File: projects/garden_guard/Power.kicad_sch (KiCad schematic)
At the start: 50 parts, among them IC1 ACPL-227-50CE, IC2 INA226AQDGSRQ1, IC3 INA226AQDGSRQ1, J7 USB_C_Receptacle_USB2.0, U10 TPS2121RUXR, U11 MAX20408AFOF, U9 Ag5810

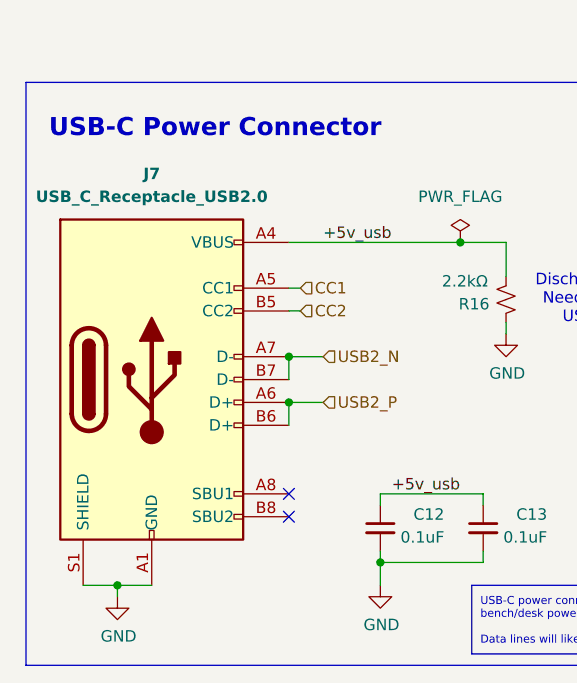
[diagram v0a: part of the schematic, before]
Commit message: - Still working through DRC - Minor board setup tweaks
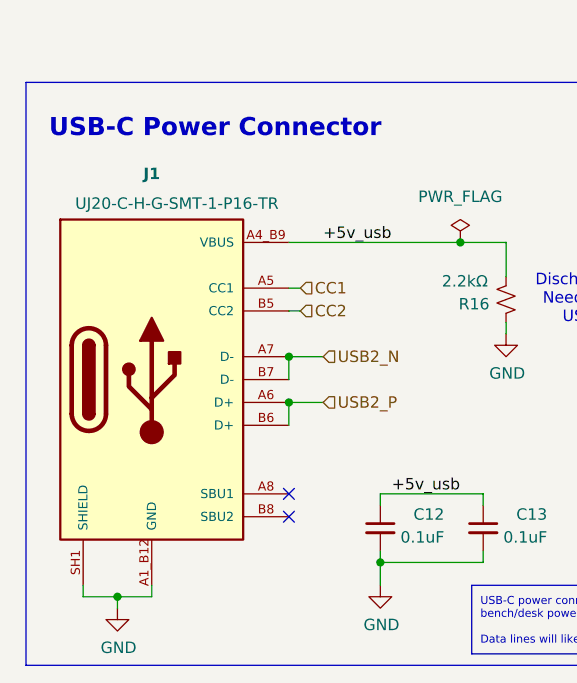
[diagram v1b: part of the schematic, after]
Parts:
- removed J7: USB_C_Receptacle_USB2.0, Connector_USB:USB_C_Receptacle_GCT_USB4105-xx-A_16P_TopMnt_Horizontal, symbol Connector:USB_C_Receptacle_USB2.0_16P
- added J1: UJ20-C-H-G-SMT-1-P16-TR, Custom_Connector:UJ20-C-H-G-SMT-1-P16-TR, symbol Custom_Connector:UJ20-C-H-G-SMT-1-P16-TR
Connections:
- net +5v_usb: now also J1.A4_B9 (VBUS), J1.B4_A9 (VBUS__1)
- net CC1: now also J1.A5 (CC1)
- net CC2: now also J1.B5 (CC2)
- net GND: now also J1.A1_B12 (GND), J1.B1_A12 (GND__1), J1.SH1 (SHIELD), J1.SH2 (SHIELD__1), J1.SH3 (SHIELD__2), J1.SH4 (SHIELD__3)
- net USB2_N: now also J1.A7 (D-), J1.B7 (D-)
- net USB2_P: now also J1.A6 (D+), J1.B6 (D+)
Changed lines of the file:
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@@
 	)
 	(junction
+		(at 24.13 177.8)
+		(diameter 0)
+		(color 0 0 0 0)
+	)
+	(junction
 		(at 162.56 142.24)
 		(diameter 0)
@@
 	)
 	(junction
-		(at 43.18 156.21)
-		(diameter 0)
-		(color 0 0 0 0)
-	)
-	(junction
 		(at 191.77 24.13)
 		(diameter 0)
@@
 	)
 	(junction
+		(at 43.18 156.21)
+		(diameter 0)
+		(color 0 0 0 0)
+	)
+	(junction
 		(at 200.66 46.99)
 		(diameter 0)
@@
 	)
 	(junction
-		(at 24.13 176.53)
+		(at 43.18 151.13)
 		(diameter 0)
 		(color 0 0 0 0)
@@
 	)
 	(junction
-		(at 43.18 151.13)
-		(diameter 0)
-		(color 0 0 0 0)
-	)
-	(junction
 		(at 137.16 49.53)
 		(diameter 0)
@@
 	(wire
 		(pts
+			(xy 24.13 179.07) (xy 24.13 177.8)
+		)
+		(stroke
+			(width 0)
+			(type default)
+		)
+	)
+	(wire
+		(pts
 			(xy 247.65 29.21) (xy 247.65 31.75)
 		)
@@
 	(wire
 		(pts
-			(xy 20.32 176.53) (xy 24.13 176.53)
+			(xy 20.32 177.8) (xy 24.13 177.8)
 		)
 		(stroke
@@
 	(wire
 		(pts
+			(xy 20.32 177.8) (xy 20.32 176.53)
+		)
+		(stroke
+			(width 0)
+			(type default)
+		)
+	)
+	(wire
+		(pts
 			(xy 93.98 34.29) (xy 97.79 34.29)
 		)
@@
 	(wire
 		(pts
+			(xy 27.94 177.8) (xy 27.94 176.53)
+		)
+		(stroke
+			(width 0)
+			(type default)
+		)
+	)
+	(wire
+		(pts
 			(xy 261.62 101.6) (xy 274.32 101.6)
 		)
@@
 	(wire
 		(pts
-			(xy 24.13 177.8) (xy 24.13 176.53)
-		)
-		(stroke
-			(width 0)
-			(type default)
-		)
-	)
-	(wire
-		(pts
 			(xy 100.33 90.17) (xy 104.14 90.17)
 		)
@@
 	(wire
 		(pts
-			(xy 24.13 176.53) (xy 27.94 176.53)
+			(xy 24.13 177.8) (xy 27.94 177.8)
 		)
 		(stroke
@@
 	(symbol
 		(lib_id "power:GND")
-		(at 24.13 177.8 0)
+		(at 24.13 179.07 0)
 		(unit 1)
 		(exclude_from_sim no)
@@
 		(dnp no)
 		(property "Reference" "#PWR034"
-			(at 24.13 184.15 0)
+			(at 24.13 185.42 0)
 			(effects
 				(font
@@
 		)
 		(property "Value" "GND"
-			(at 24.257 182.1942 0)
+			(at 24.257 183.4642 0)
 			(effects
 				(font
@@
 		)
 		(property "Footprint" ""
-			(at 24.13 177.8 0)
+			(at 24.13 179.07 0)
 			(effects
 				(font
@@
 		)
 		(property "Datasheet" ""
-			(at 24.13 177.8 0)
+			(at 24.13 179.07 0)
 			(effects
 				(font
@@
 		)
 		(property "Description" "Power symbol creates a global label with name \"GND\" , ground"
-			(at 24.13 177.8 0)
+			(at 24.13 179.07 0)
 			(effects
 				(font
@@
 	)
 	(symbol
-		(lib_id "Connector:USB_C_Receptacle_USB2.0_16P")
-		(at 27.94 153.67 0)
+		(lib_id "Custom_Connector:UJ20-C-H-G-SMT-1-P16-TR")
+		(at 27.94 154.94 0)
 		(unit 1)
 		(exclude_from_sim no)
@@
 		(on_board yes)
 		(dnp no)
-		(fields_autoplaced yes)
-		(property "Reference" "J7"
+		(property "Reference" "J1"
 			(at 27.94 130.81 0)
 			(effects
@@
 			)
 		)
-		(property "Value" "USB_C_Receptacle_USB2.0"
-			(at 27.94 133.35 0)
-			(effects
-				(font
-					(size 1.27 1.27)
-					(thickness 0.254)
-					(bold yes)
-				)
-			)
-		)
-		(property "Footprint" "Connector_USB:USB_C_Receptacle_GCT_USB4105-xx-A_16P_TopMnt_Horizontal"
-			(at 31.75 153.67 0)
-			(effects
-				(font
-					(size 1.27 1.27)
-				)
-				(hide yes)
-			)
-		)
-		(property "Datasheet" "https://www.usb.org/sites/default/files/documents/usb_type-c.zip"
-			(at 31.75 153.67 0)
+		(property "Value" "UJ20-C-H-G-SMT-1-P16-TR"
+			(at 30.734 134.112 0)
 			(effects
 				(font
 					(size 1.27 1.27)
 				)
-				(hide yes)
 			)
 		)
-		(property "Description" "USB 2.0-only 16P Type-C Receptacle connector"
-			(at 27.94 153.67 0)
-			(effects
-				(font
-					(size 1.27 1.27)
-				)
-				(hide yes)
-			)
-		)
-		(property "MPN" "UJ20-C-H-G-SMT-1-P16-TR"
-			(at 27.94 153.67 0)
+		(property "Footprint" "Custom_Connector:UJ20-C-H-G-SMT-1-P16-TR"
+			(at 127 160.02 0)
 			(effects
 				(font
 					(size 1.27 1.27)
 				)
+				(justify bottom)
 				(hide yes)
 			)
 		)
-		(property "Mfr" "Same Sky"
-			(at 27.94 153.67 0)
+		(property "Datasheet" ""
+			(at 27.94 160.02 0)
 			(effects
 				(font
@@
 			)
 		)
-		(property "JLCPCB_PN" "C45082766"
-			(at 27.94 153.67 0)
+		(property "Description" ""
+			(at 27.94 160.02 0)
 			(effects
 				(font
@@
 			)
 		)
-		(property "Class" "connector"
-			(at 27.94 153.67 0)
+		(property "PARTREV" "1.0"
+			(at 27.94 158.75 0)
 			(effects
 				(font
 					(size 1.27 1.27)
 				)
+				(justify bottom)
 				(hide yes)
 			)
 		)
-		(property "Critical" "yes"
-			(at 27.94 153.67 0)
+		(property "MANUFACTURER" "Same Sky"
+			(at 73.66 152.4 0)
 			(effects
 				(font
 					(size 1.27 1.27)
 				)
+				(justify bottom)
 				(hide yes)
 			)
 		)
-		(property "Dielectric_Class" ""
-			(at 27.94 153.67 0)
+		(property "MAXIMUM_PACKAGE_HEIGHT" "3.46mm"
+			(at 73.66 152.4 0)
 			(effects
 				(font
 					(size 1.27 1.27)
 				)
+				(justify bottom)
 				(hide yes)
 			)
 		)
-		(property "Color" ""
-			(at 27.94 153.67 0)
+		(property "STANDARD" "Manufacturer Recommendations"
+			(at 73.66 152.4 0)
 			(effects
 				(font
 					(size 1.27 1.27)
 				)
+				(justify bottom)
 				(hide yes)
 			)
 		)
-		(pin "A1"
-		)
-		(pin "A12"
+		(pin "B5"
 		)
-		(pin "A4"
+		(pin "B1_A12"
 		)
-		(pin "A5"
+		(pin "A8"
 		)
 		(pin "A6"
 		)
-		(pin "A7"
+		(pin "B8"
 		)
-		(pin "A8"
+		(pin "SH4"
 		)
-		(pin "A9"
+		(pin "B4_A9"
 		)
-		(pin "B1"
+		(pin "B6"
 		)
-		(pin "B12"
+		(pin "SH2"
 		)
-		(pin "B4"
+		(pin "A4_B9"
 		)
-		(pin "B5"
+		(pin "SH3"
 		)
-		(pin "B6"
+		(pin "A1_B12"
 		)
-		(pin "B7"
+		(pin "A5"
 		)
-		(pin "B8"
+		(pin "SH1"
 		)
-		(pin "B9"
+		(pin "B7"
 		)
-		(pin "S1"
+		(pin "A7"
 		)
 		(instances
-			(project "garden_guard"
+			(project ""
 				(path "/dcdac9d4-ef08-426f-b97c-7b9219501e71/446b5b12-2582-472d-9a1e-c1c7d43f42d1"
-					(reference "J7")
+					(reference "J1")
 					(unit 1)
 				)
